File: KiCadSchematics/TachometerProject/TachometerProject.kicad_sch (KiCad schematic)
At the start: 2 parts

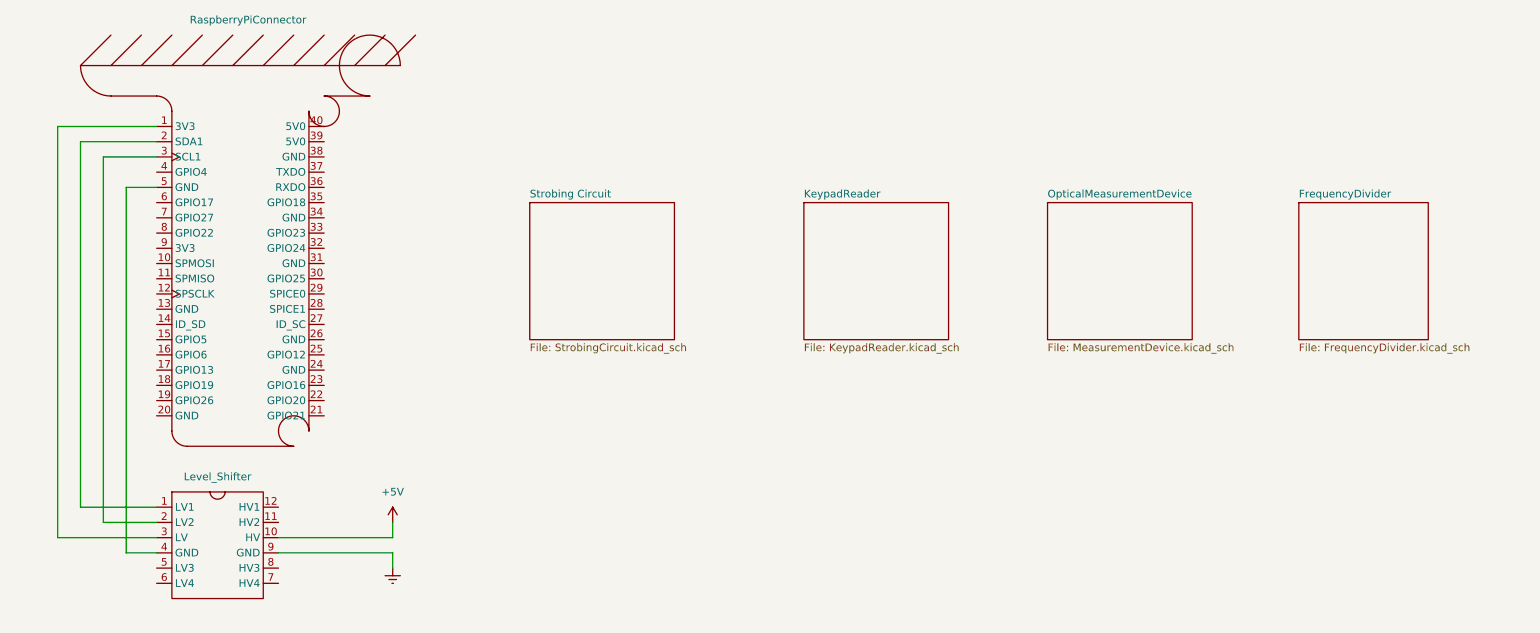
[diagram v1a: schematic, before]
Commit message: Updated Schematic Drawings, README
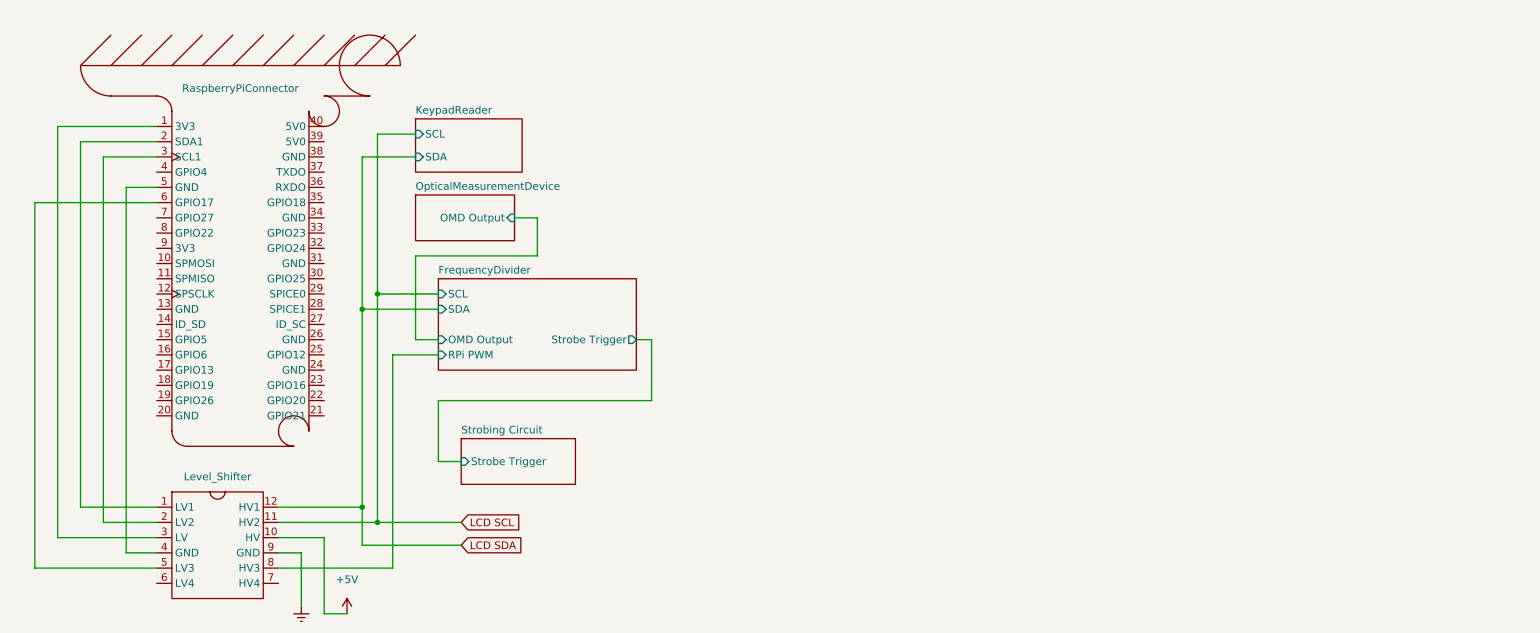
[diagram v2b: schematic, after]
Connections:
- net LCD SCL: now reaches U?.11 (HV2)
- net LCD SDA: now reaches U?.12 (HV1)
- net at U?.5 (LV3): now also U?.6 (GPIO17)
- net FrequencyDivider/RPi PWM: now reaches U?.8 (HV3)
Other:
- sheet FrequencyDivider ports: added OMD Output, RPi PWM, SCL, SDA, Strobe Trigger; removed none
- sheet KeypadReader ports: added SCL, SDA; removed none
- sheet OpticalMeasurementDevice ports: added OMD Output; removed none
- sheet Strobing Circuit ports: added Strobe Trigger; removed none

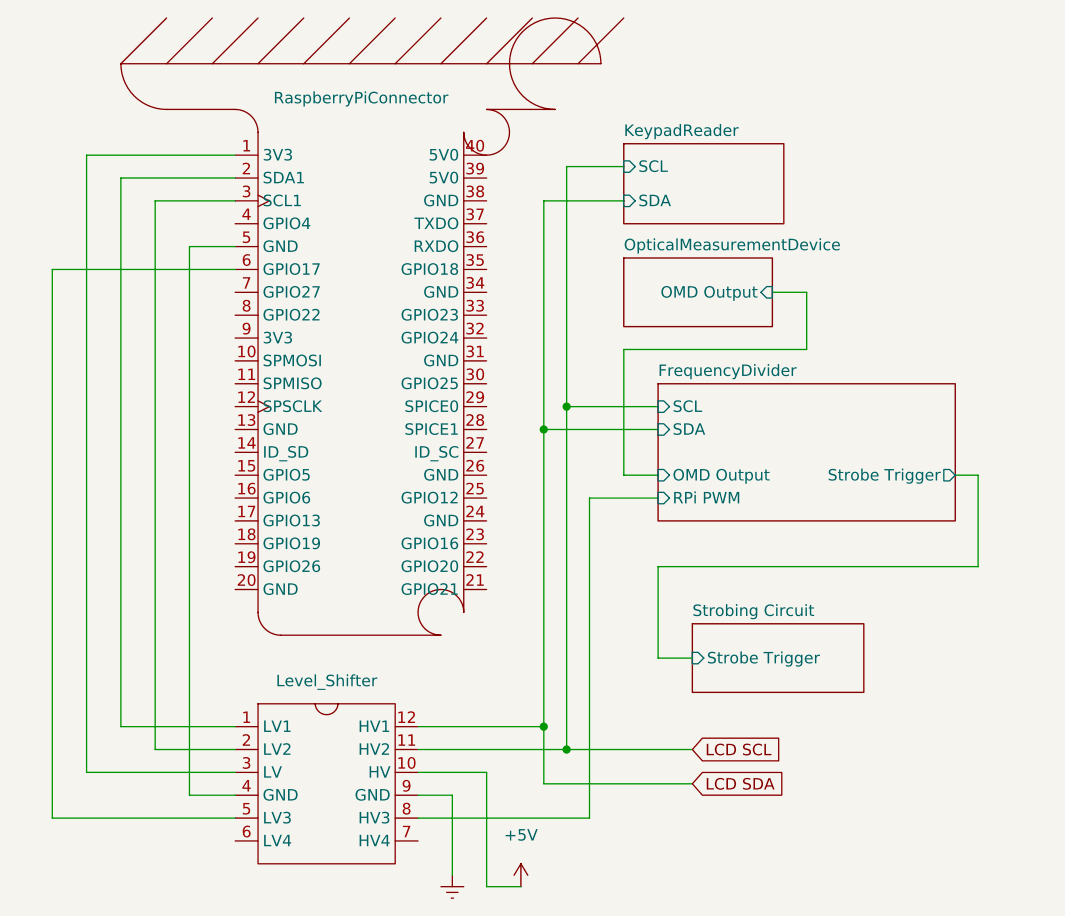
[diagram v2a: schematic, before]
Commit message: Updated circuit diagrams
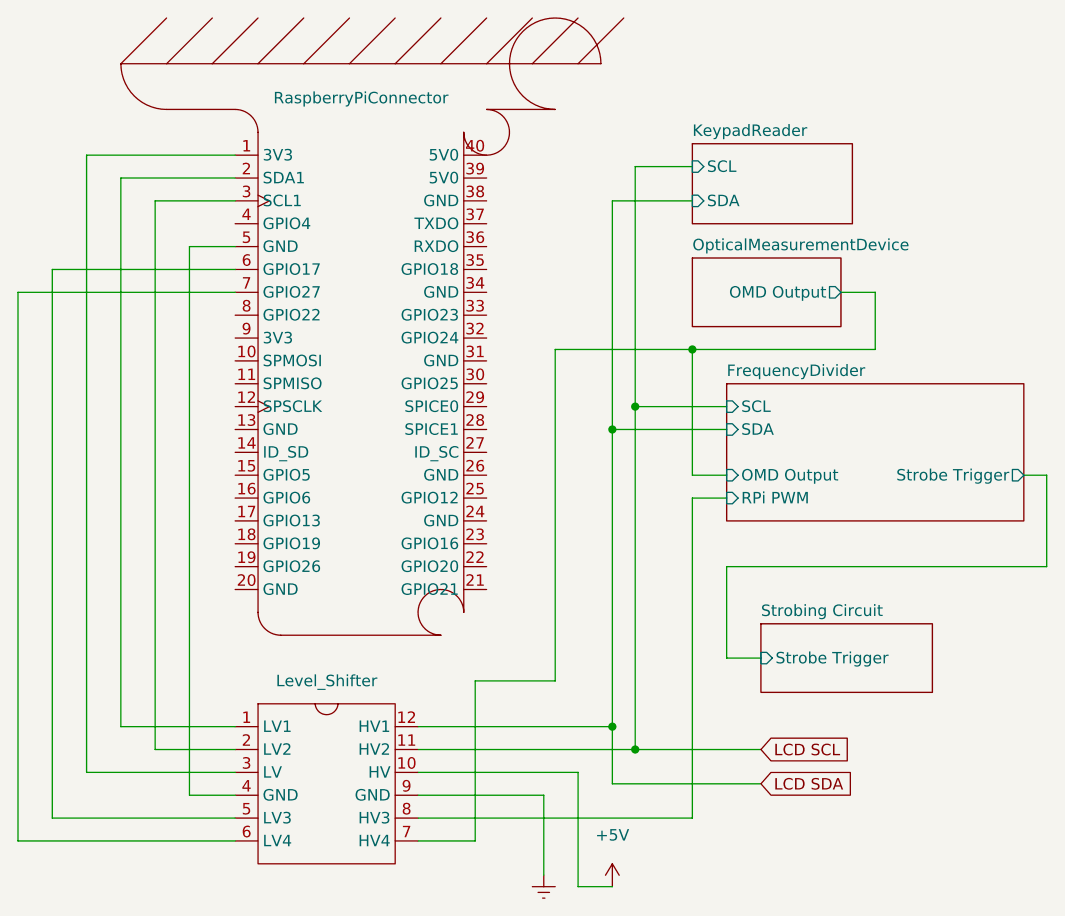
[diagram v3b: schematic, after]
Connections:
- net FrequencyDivider/OMD Output: now also U?.7 (HV4)
- net at U?.6 (LV4): now also U?.7 (GPIO27)
